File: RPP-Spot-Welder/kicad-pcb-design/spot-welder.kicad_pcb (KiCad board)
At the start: 2 copper layers, 18 parts, among them J1 Encoder1, J2 ST7789V Connector, J3 20x4 Connector, J4 100F 16V Super Cap, J5 Weld Pin -, J6 Relay, U1 Pico

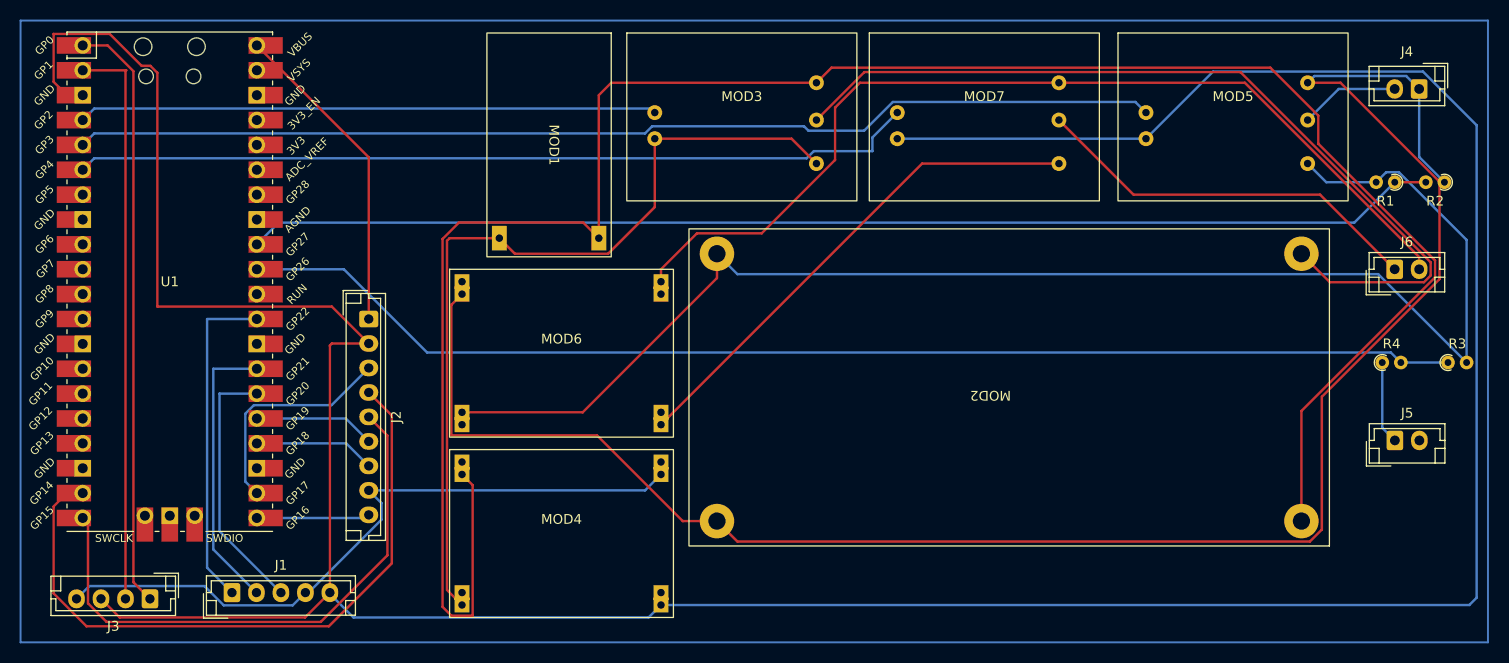
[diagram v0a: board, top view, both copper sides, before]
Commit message: update the design
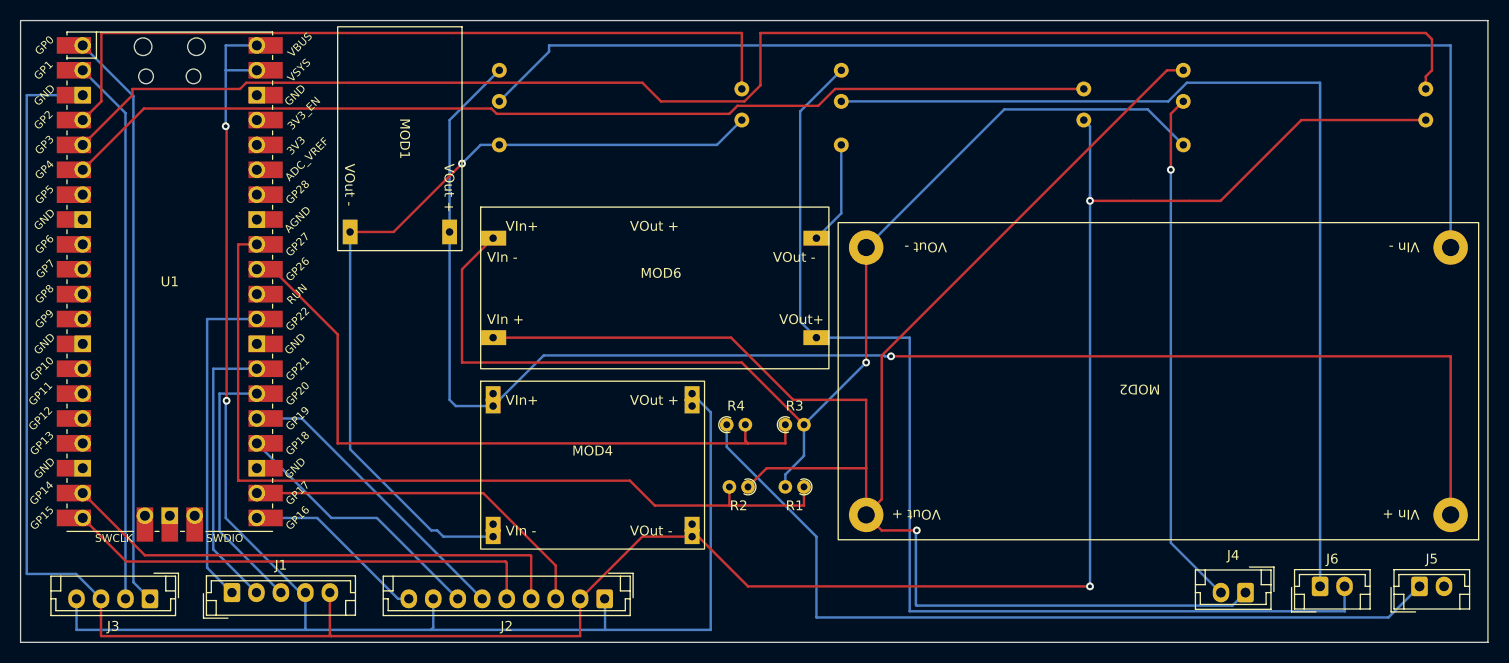
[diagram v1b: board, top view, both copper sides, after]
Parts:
- MOD3, MOD5, MOD7: moved to B.Cu
- MOD6: footprint Custom_Modules:BUCK_COVERTER -> Custom_Modules:BOOST_COVERTER
- moved R2 77.6 mm to (87.0, 60.3)
- moved R3 68.0 mm to (90.8, 54.0)
- moved R1 67.9 mm to (92.7, 60.3)
- moved R4 67.2 mm to (84.8, 54.0)
- moved J4 54.4 mm to (137.8, 71.1)
- moved J2 37.4 mm to (72.3, 71.8), turned to 180 degrees
- moved J6 33.3 mm to (145.4, 70.5)
- moved MOD1 15.3 mm to (51.4, 24.8)
- moved MOD2 15.3 mm to (127.0, 49.8)
- moved J5 15.1 mm to (155.6, 70.5)
- moved MOD5 12.8 mm to (149.2, 19.7), turned to 180 degrees
- moved MOD4 7.67 mm to (71.1, 57.1)
- moved MOD6 7.10 mm to (71.1, 39.4)
- moved MOD3 7.10 mm to (79.4, 19.7), turned to 180 degrees
- moved MOD7 3.42 mm to (114.3, 19.7), turned to 180 degrees
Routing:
- net Net-(J1-Pin_5): track 352.1 -> 267.3 mm, vias 0 -> 2
- net Net-(J5-Pin_1): track 8.49 -> 86.4 mm
- net +3.3V: track 102.5 -> 168.8 mm, vias 0 -> 2
- net Net-(J6-Pin_1): track 40.6 -> 101.1 mm
- net VCC: track 216.5 -> 156.6 mm, vias 0 -> 1
- net Net-(U1-GPIO26_ADC0): track 125.6 -> 70.2 mm
- net Net-(J4-Pin_2): track 10.2 -> 52.8 mm, vias 0 -> 1
- net Net-(MOD5-Trigger+): track 111.2 -> 153.2 mm
- net Net-(MOD6-VOut-): track 51.7 -> 10.6 mm
- net Net-(U1-GPIO27_ADC1): track 122.0 -> 88.7 mm
- net Net-(MOD2-Vin-): track 88.8 -> 120.5 mm
- net Net-(MOD2-Vout-): track 148.2 -> 119.2 mm, vias 0 -> 1
- net Net-(MOD3-Trigger+): track 58.5 -> 80.8 mm
- net Net-(MOD7-Trigger+): track 86.4 -> 106.1 mm
- net Net-(J2-Pin_6): track 12.4 -> 30.6 mm
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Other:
- board outline added: 149.9 x 63.5 mm
